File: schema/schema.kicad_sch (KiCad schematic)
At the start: 13 parts, among them J1 Conn_01x15, J2 Conn_01x15, J3 Conn_01x15, J4 Conn_01x15, J5 Conn_01x03, SW1 SW_Push, SW2 SW_Push, SW3 SW_Push

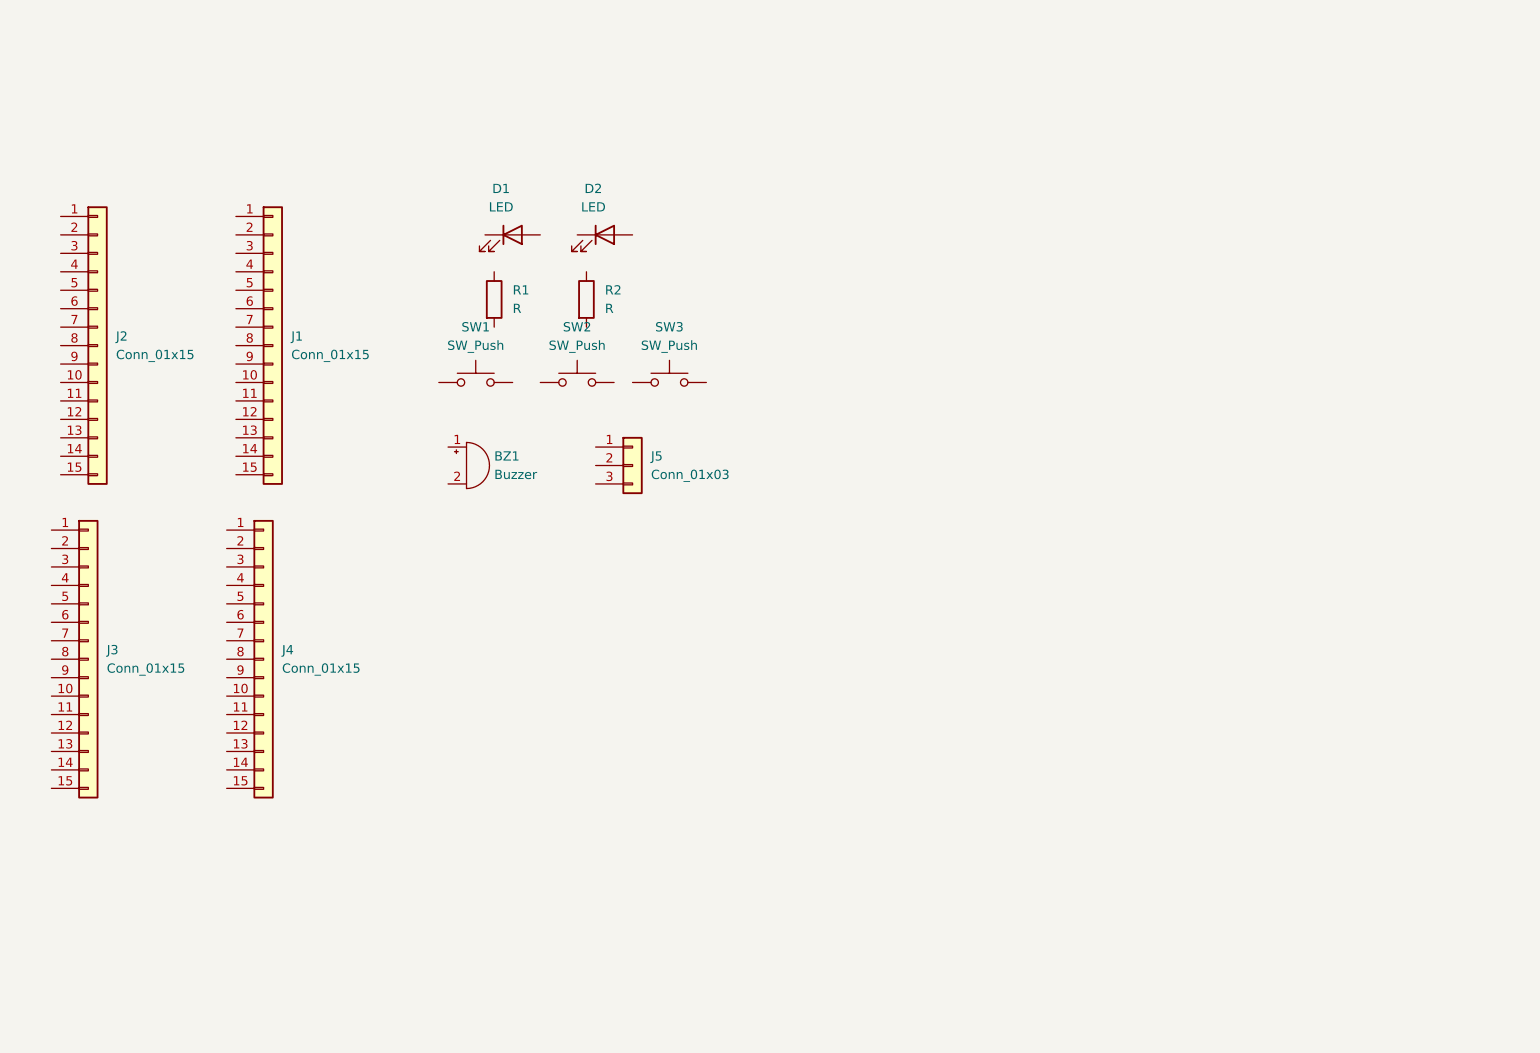
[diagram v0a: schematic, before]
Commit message: Finish transmitter-board schema
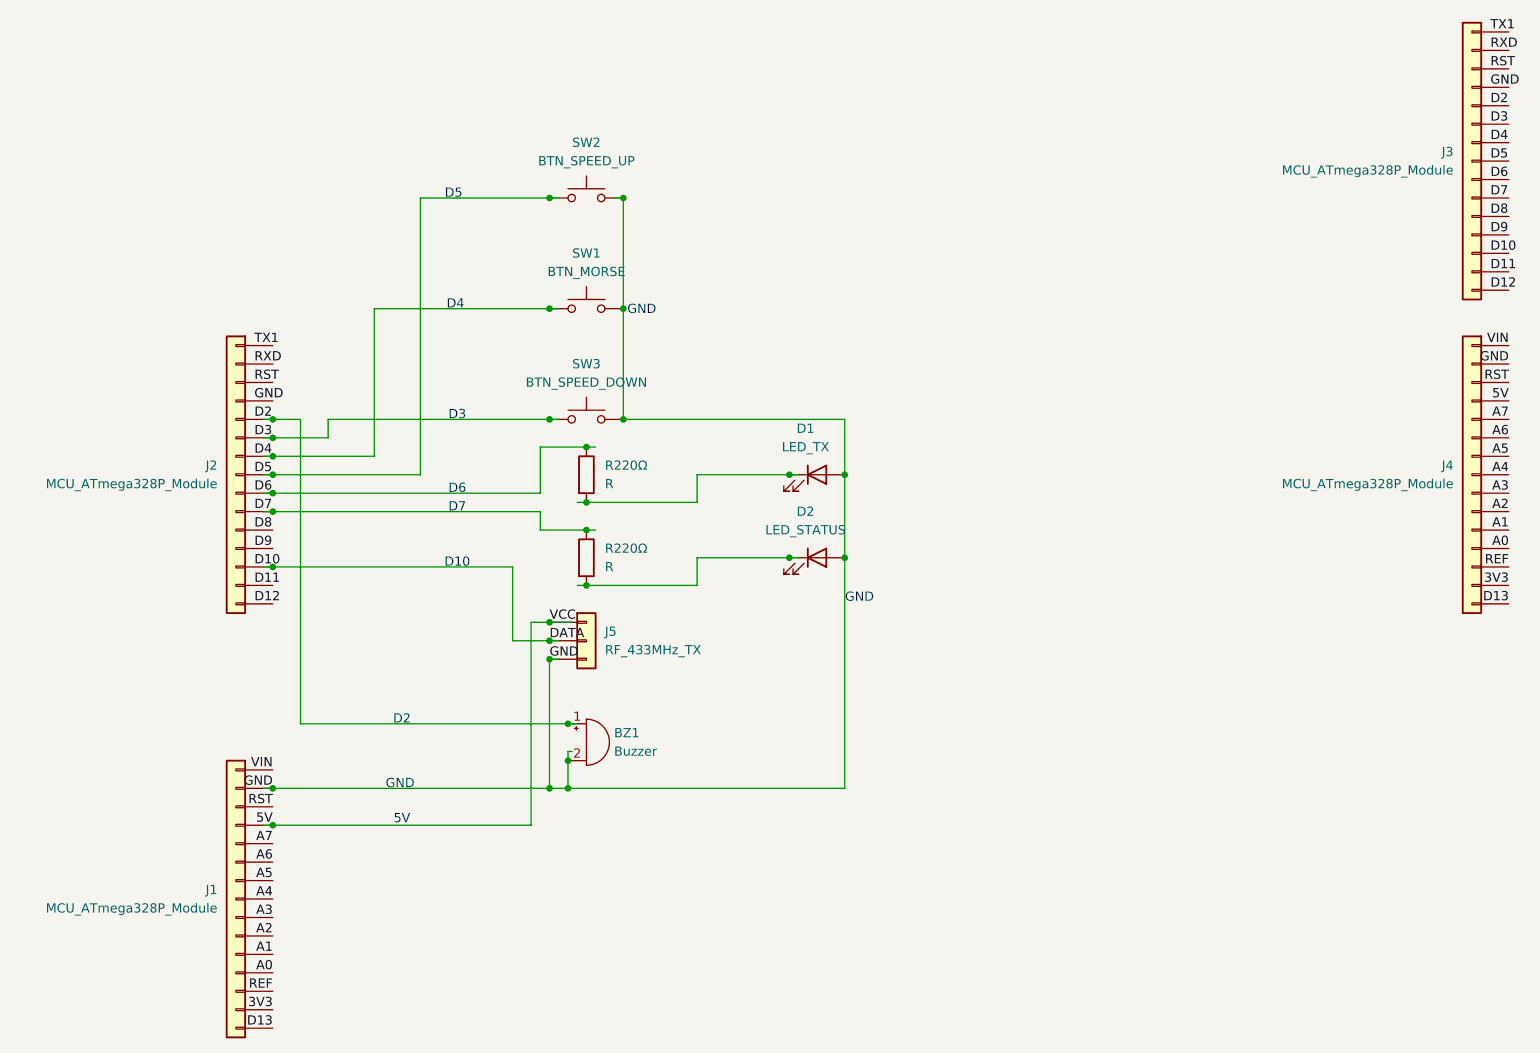
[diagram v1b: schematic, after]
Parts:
- D1: value LED -> LED_TX
- D2: value LED -> LED_STATUS
- J1, J2, J3, J4: value Conn_01x15 -> MCU_ATmega328P_Module
- J5: value Conn_01x03 -> RF_433MHz_TX
- SW1: value SW_Push -> BTN_MORSE
- SW2: value SW_Push -> BTN_SPEED_UP
- SW3: value SW_Push -> BTN_SPEED_DOWN
- renumbered R1 to R220Ω, R2 to R220Ω
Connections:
- net at D1.1 (K): now also R220Ω.2
- net GND: now reaches D1.2 (A)
- net GND: now also BZ1.2 (-), D2.2 (A), J1.2 (Pin_2), J4.2 (Pin_2), J5.3 (Pin_3), SW1.2, SW2.2, SW3.2
- net at SW2.1: now also J2.8 (Pin_8)
- net at D2.1 (K): now also R220Ω.2
- net at J2.10 (Pin_10): now also R220Ω.1
- net DATA: now reaches J2.13 (Pin_13)
- net DATA: now also J5.2 (Pin_2)
- net at J2.5 (Pin_5): now also BZ1.1 (+)
- net at J2.6 (Pin_6): now also SW3.1
- net at J2.7 (Pin_7): now also SW1.1
- net at J2.9 (Pin_9): now also R220Ω.1
- net 5V: now reaches J5.1 (Pin_1)
- net 5V: now also J1.4 (Pin_4), J4.4 (Pin_4)
- net VIN: now reaches J4.1 (Pin_1)
- net VIN: now also J1.1 (Pin_1)
- net A2: now reaches J4.10 (Pin_10)
- net A2: now also J1.10 (Pin_10)
- net A1: now reaches J4.11 (Pin_11)
- net A1: now also J1.11 (Pin_11)
- net A0: now reaches J4.12 (Pin_12)
- net A0: now also J1.12 (Pin_12)
- net REF: now reaches J4.13 (Pin_13)
- net REF: now also J1.13 (Pin_13)
- net 3V3: now reaches J4.14 (Pin_14)
- net 3V3: now also J1.14 (Pin_14)
- net D13: now reaches J4.15 (Pin_15)
- net D13: now also J1.15 (Pin_15)
- net RST: now reaches J4.3 (Pin_3)
- net RST: now also J1.3 (Pin_3)
- net A7: now reaches J4.5 (Pin_5)
- net A7: now also J1.5 (Pin_5)
- net A6: now reaches J4.6 (Pin_6)
- net A6: now also J1.6 (Pin_6)
- net A5: now reaches J4.7 (Pin_7)
- net A5: now also J1.7 (Pin_7)
- net A4: now reaches J4.8 (Pin_8)
- net A4: now also J1.8 (Pin_8)
- net A3: now reaches J4.9 (Pin_9)
- net A3: now also J1.9 (Pin_9)
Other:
- note added: "5V"
- note added: "D10"
- note added: "D2"
- note added: "D3"
- note added: "D4"
- note added: "D5"
- note added: "D6"
- note added: "D7"
- note added: "GND"
- moved on the sheet: D1, D2, R220Ω, SW1, SW2, SW3
